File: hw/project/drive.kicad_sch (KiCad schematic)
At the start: 63 parts, among them Q10 STL110N10F7, Q5 STL110N10F7, Q6 STL110N10F7, Q7 STL110N10F7, Q8 STL110N10F7, Q9 STL110N10F7

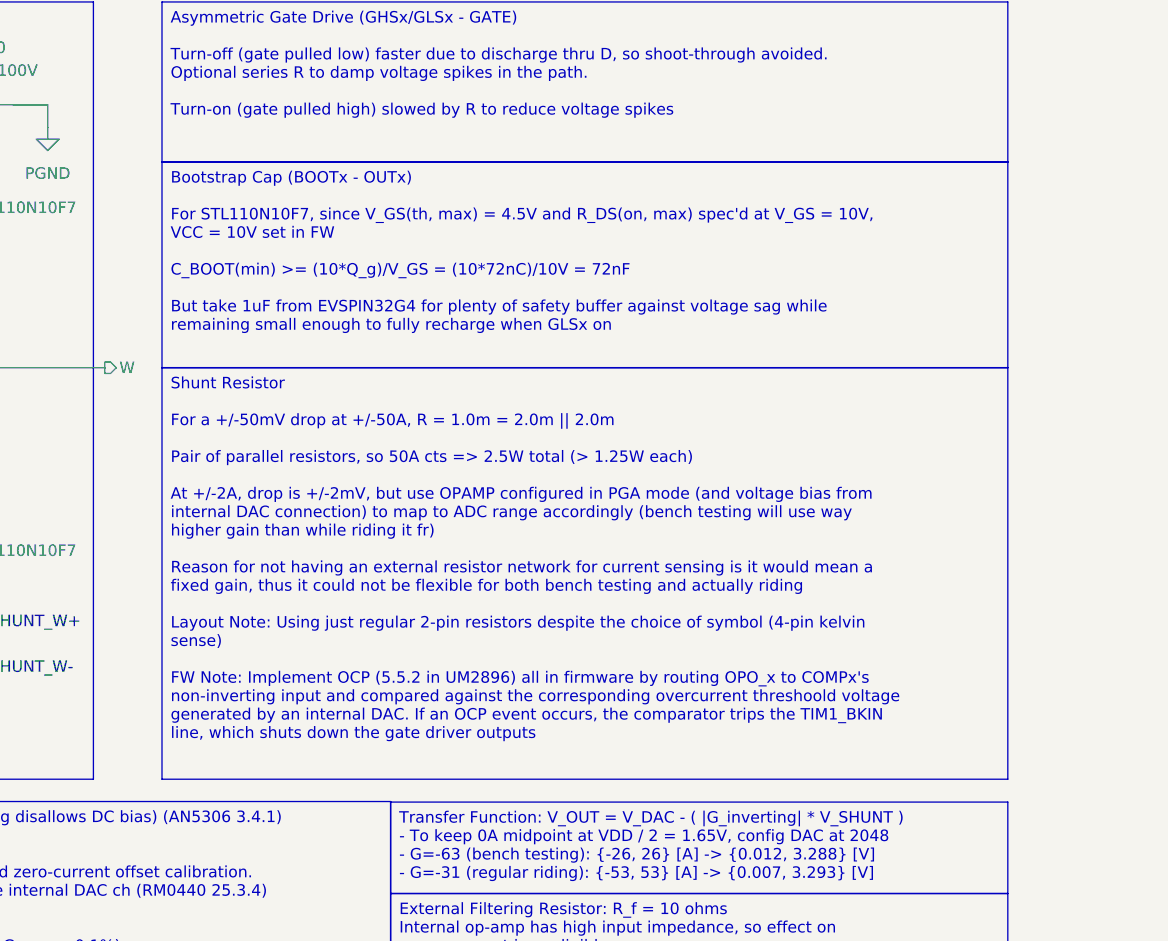
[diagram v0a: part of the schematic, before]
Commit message: Continuing power revamp tomorrow
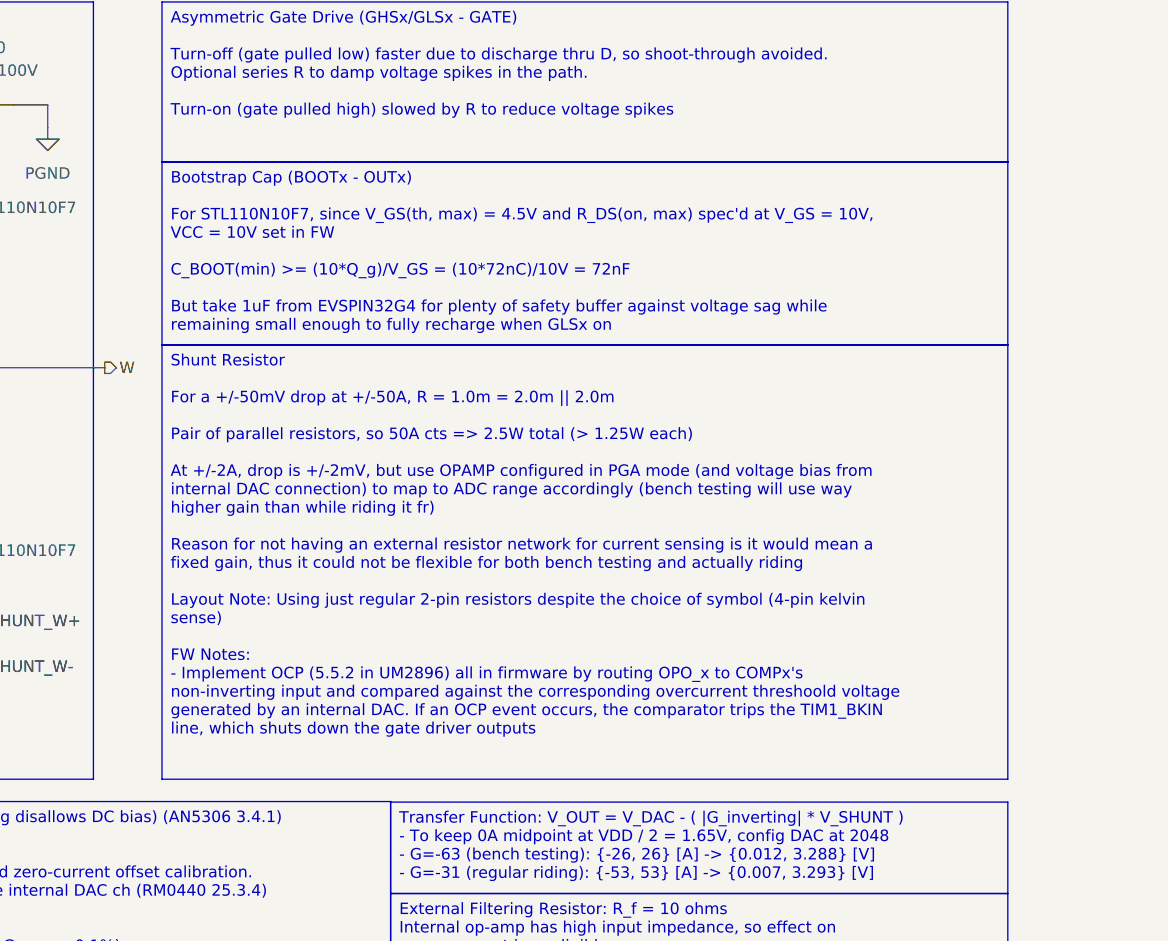
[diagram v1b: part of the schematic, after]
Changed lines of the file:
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@@
 		(exclude_from_sim no)
 		(at 220.98 38.1001 0)
-		(size 93.98 22.8453)
+		(size 93.98 20.3199)
 		(margins 0.9525 0.9525 0.9525 0.9525)
 		(stroke
@@
 		)
 	)
-	(text_box "Shunt Resistor\n\nFor a +/-50mV drop at +/-50A, R = 1.0m = 2.0m || 2.0m\n\nPair of parallel resistors, so 50A cts => 2.5W total (> 1.25W each)\n\nAt +/-2A, drop is +/-2mV, but use OPAMP configured in PGA mode (and voltage bias from internal DAC connection) to map to ADC range accordingly (bench testing will use way higher gain than while riding it fr)\n\nReason for not having an external resistor network for current sensing is it would mean a fixed gain, thus it could not be flexible for both bench testing and actually riding\n\nLayout Note: Using just regular 2-pin resistors despite the choice of symbol (4-pin kelvin sense)\n\nFW Note: Implement OCP (5.5.2 in UM2896) all in firmware by routing OPO_x to COMPx's non-inverting input and compared against the corresponding overcurrent threshoold voltage generated by an internal DAC. If an OCP event occurs, the comparator trips the TIM1_BKIN line, which shuts down the gate driver outputs"
+	(text_box "Shunt Resistor\n\nFor a +/-50mV drop at +/-50A, R = 1.0m = 2.0m || 2.0m\n\nPair of parallel resistors, so 50A cts => 2.5W total (> 1.25W each)\n\nAt +/-2A, drop is +/-2mV, but use OPAMP configured in PGA mode (and voltage bias from internal DAC connection) to map to ADC range accordingly (bench testing will use way higher gain than while riding it fr)\n\nReason for not having an external resistor network for current sensing is it would mean a fixed gain, thus it could not be flexible for both bench testing and actually riding\n\nLayout Note: Using just regular 2-pin resistors despite the choice of symbol (4-pin kelvin sense)\n\nFW Notes: \n- Implement OCP (5.5.2 in UM2896) all in firmware by routing OPO_x to COMPx's non-inverting input and compared against the corresponding overcurrent threshoold voltage generated by an internal DAC. If an OCP event occurs, the comparator trips the TIM1_BKIN line, which shuts down the gate driver outputs"
 		(exclude_from_sim no)
-		(at 220.98 60.9601 0)
-		(size 93.98 45.7199)
+		(at 220.98 58.4199 0)
+		(size 93.98 48.2601)
 		(margins 0.9525 0.9525 0.9525 0.9525)
 		(stroke
